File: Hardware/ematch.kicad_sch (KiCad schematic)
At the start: 41 parts, among them J3 Conn_01x02_Male, J4 Conn_01x02_Male, J5 Conn_01x02_Male, J6 Conn_01x02_Male, Q1 BSZ025N04LS, Q2 BSZ025N04LS, Q3 BSZ025N04LS, Q4 BSZ025N04LS, U6 LTV-247

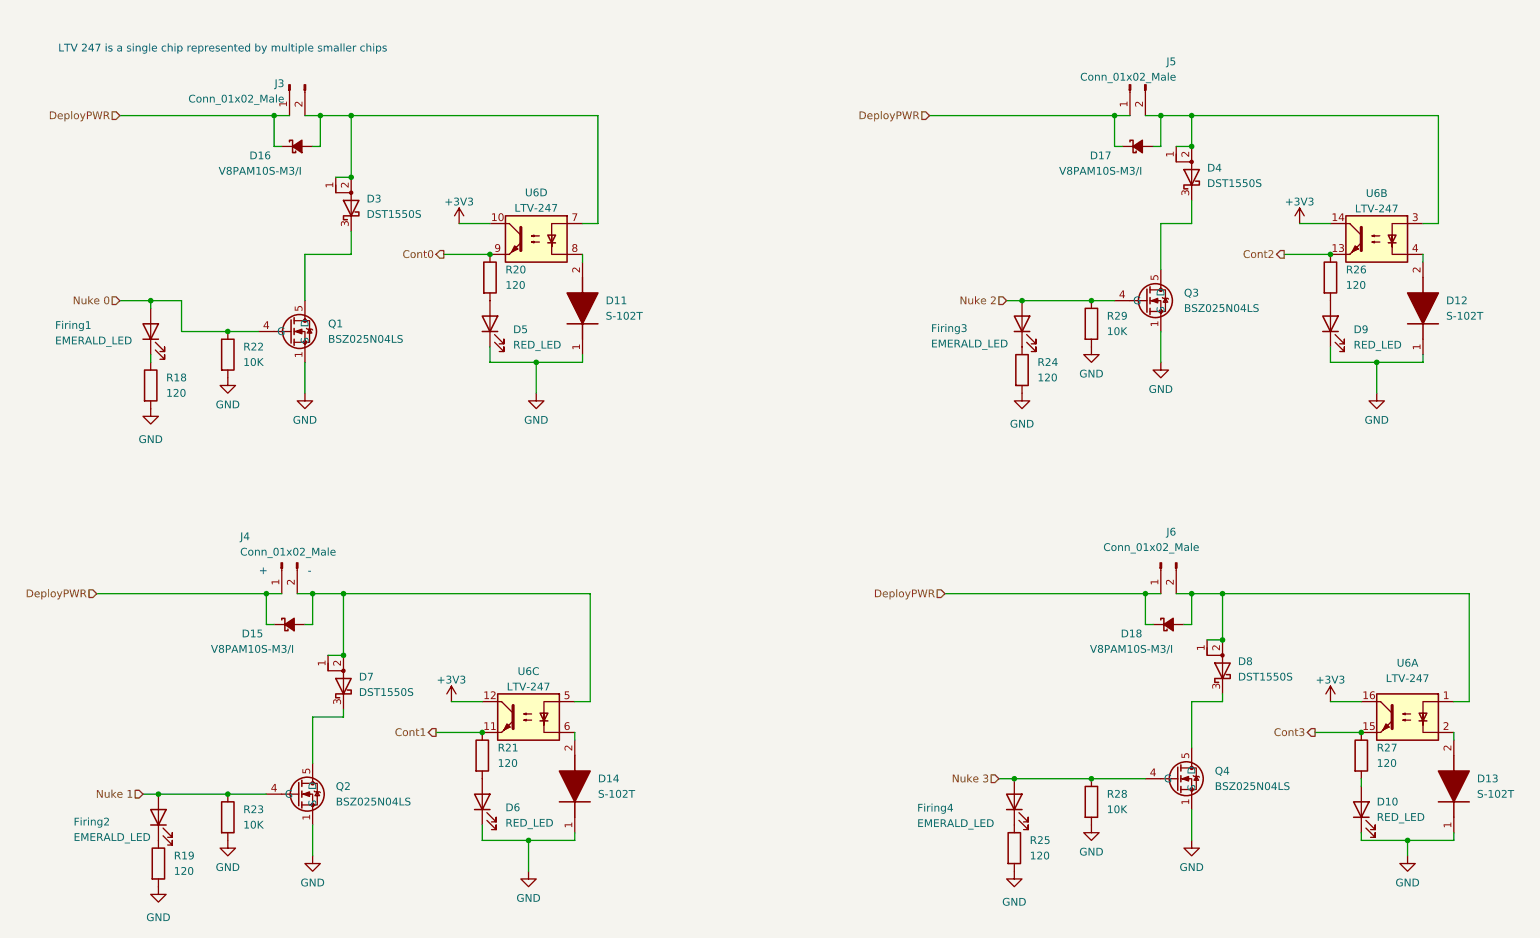
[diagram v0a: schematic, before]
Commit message: files
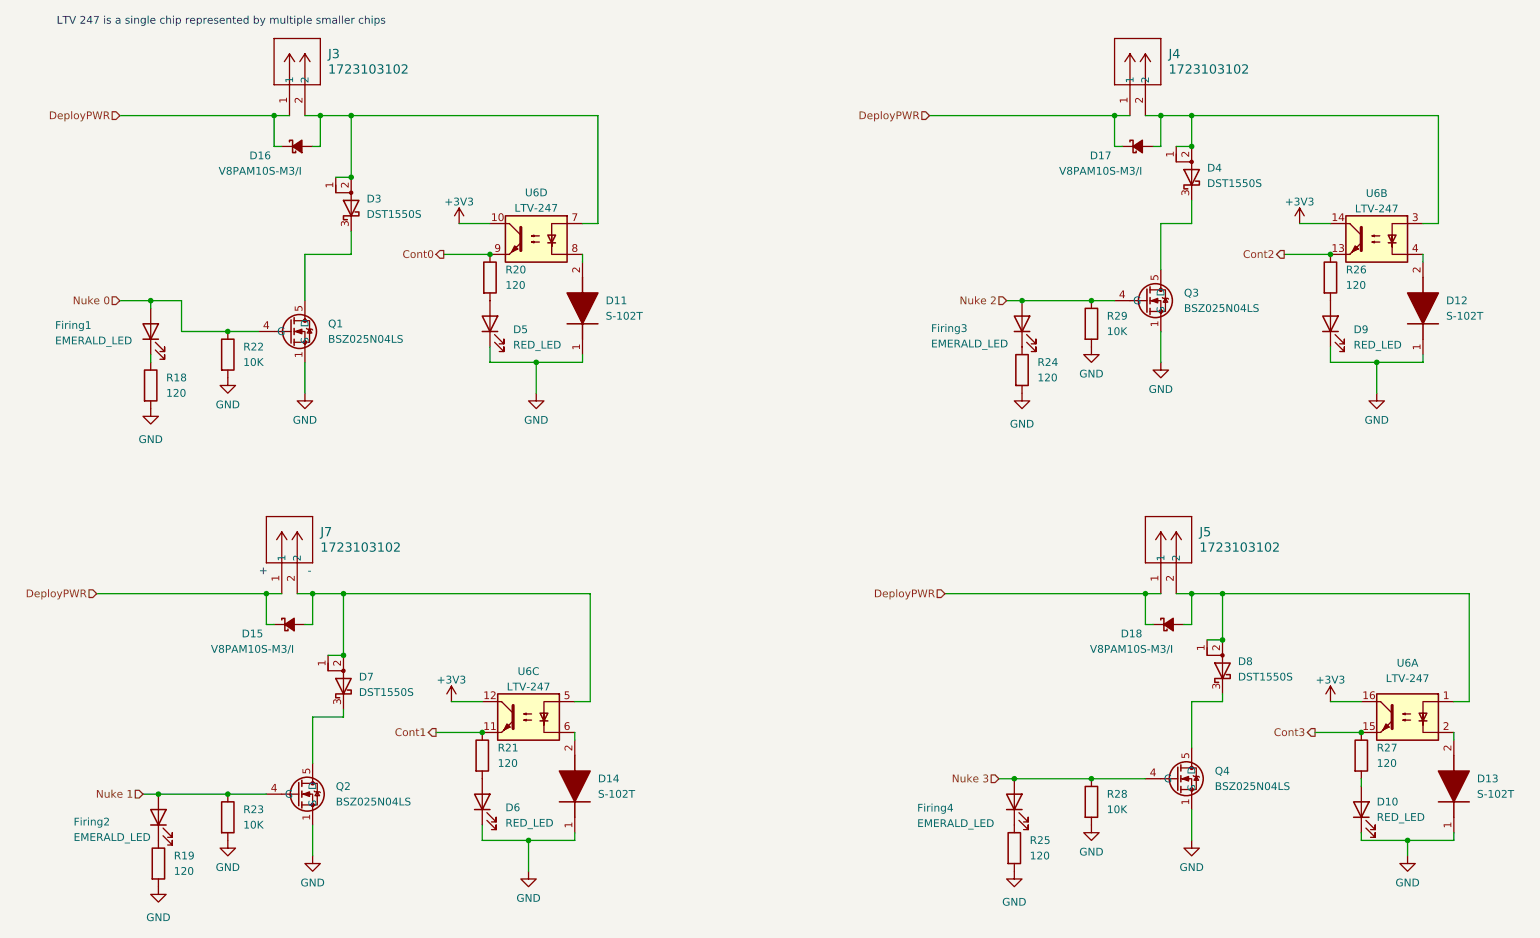
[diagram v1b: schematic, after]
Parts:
- removed J3, J4, J5, J6: Conn_01x02_Male, TerminalBlock_Phoenix:TerminalBlock_Phoenix_PT-1,5-2-3.5-H_1x02_P3.50mm_Horizontal, symbol Connector:Conn_01x02_Male
- added J3, J4, J5, J7: 1723103102, iclr:CONN_1723102000_02_MOL, symbol ICLR_HW:1723103102
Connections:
- net DeployPWR: now also J3.1, J4.1, J5.1, J7.1
- net at D16.2 (A), D3.1 (A), D3.2 (A)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: now also J3.2
- net at D18.2 (A), D8.1 (A), D8.2 (A)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: now also J5.2
- net at D15.2 (A), D7.1 (A), D7.2 (A)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: now also J7.2
- net at D17.2 (A), D4.1 (A), D4.2 (A)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: now also J4.2
